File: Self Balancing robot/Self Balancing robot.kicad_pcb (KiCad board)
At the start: 2 copper layers, 90 x 60 mm, 14 parts, among them J1 TB002-500-02BE, J5 TB002-500-03BE, J7 SSK01-MPH-254-A4, J8 SSK01-MPH-254-A4, U1 ESP32-DEVKIT-V1, U2 GY-521

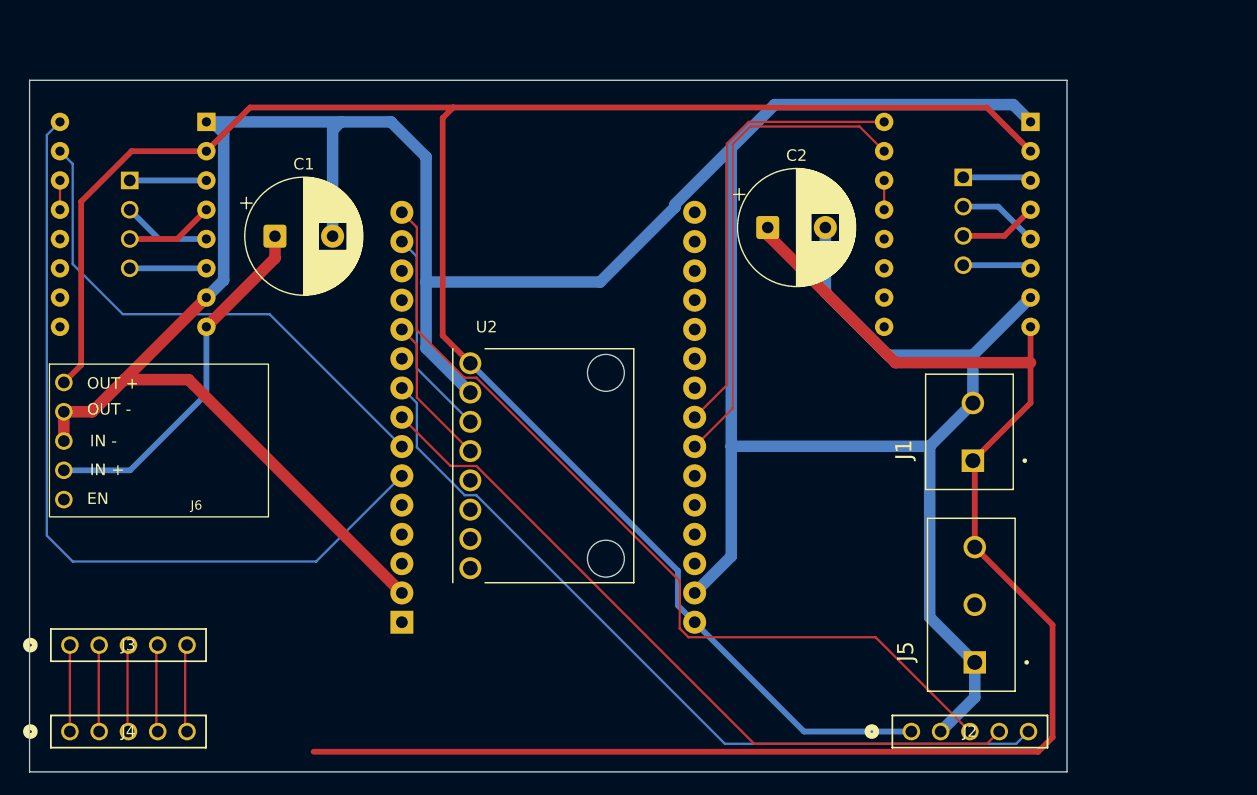
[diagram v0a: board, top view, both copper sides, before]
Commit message: In progress commit (Will fix on laptop)
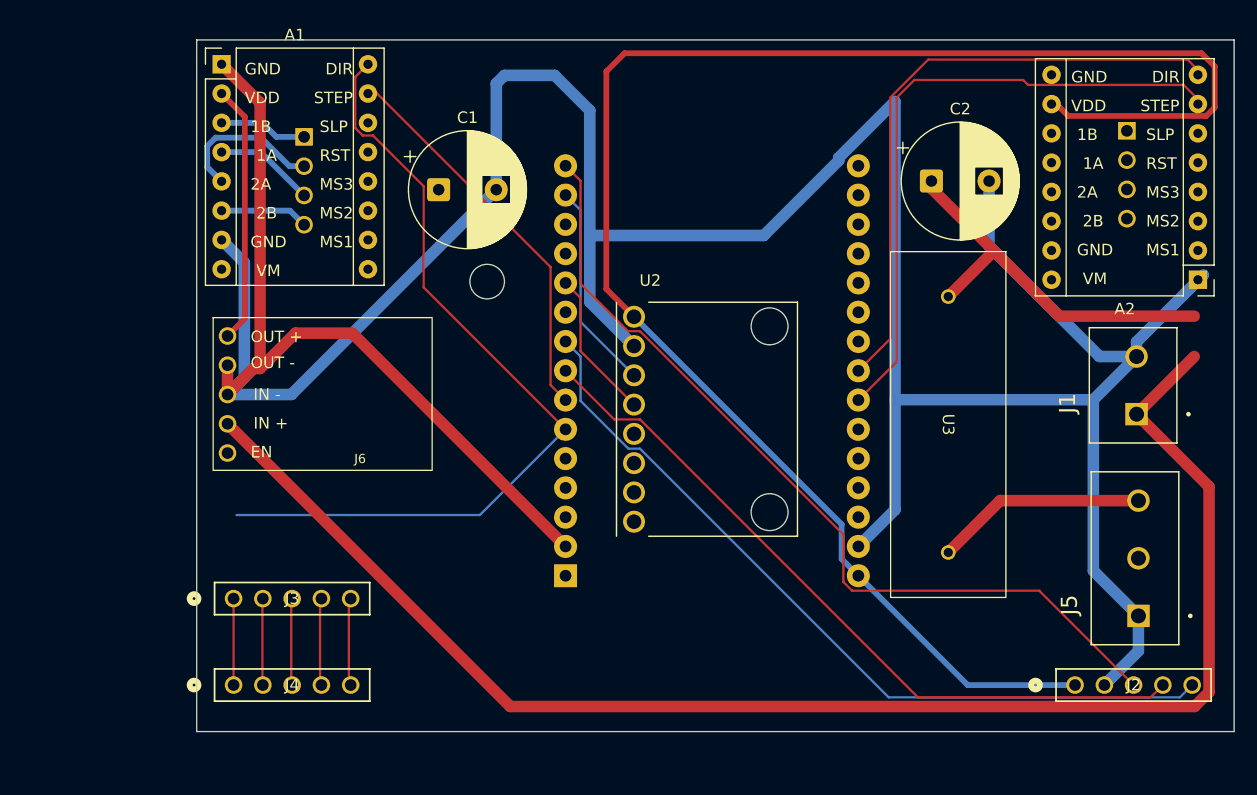
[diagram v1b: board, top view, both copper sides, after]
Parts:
- added U3: ~, 5A Fuse:5A Fuse, F.Cu at (170.2, 118.4)
- A1, A2: moved to F.Cu
- moved J7 15.6 mm to (109.3, 112.2)
- moved U2 14.8 mm to (144.3, 132.9)
- moved J3 14.8 mm to (103.2, 148.5)
- moved J4 14.8 mm to (103.2, 156.0)
- moved J6 14.8 mm to (98.2, 132.3)
- moved C1 14.8 mm to (121.0, 113.0)
- moved C2 14.8 mm to (163.7, 112.2)
- moved J8 14.8 mm to (180.7, 111.7)
- moved J1 14.8 mm to (181.5, 132.5)
- moved J2 14.8 mm to (176.2, 156.0)
- moved J5 14.8 mm to (181.7, 150.0)
- moved U1 14.8 mm to (144.7, 131.0)
- moved A1 5.17 mm to (102.2, 102.1), turned to 0 degrees
- moved A2 4.76 mm to (174.4, 102.8), turned to 0 degrees
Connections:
- J5 pad 3: +7.5V -> Net-(U3-Input)
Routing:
- net Net-(U3-Input): track 0.00 -> 18.4 mm
- net Net-(A2-DIR): track 39.3 -> 53.6 mm
- net Net-(A2-STEP): track 42.2 -> 55.4 mm
- net Net-(A1-STEP): track 45.4 -> 34.2 mm
- net +5V: track 180.4 -> 170.3 mm
- net GND: track 301.6 -> 309.3 mm
- net Net-(A2-2A): track 7.00 -> 0.00 mm
- net Net-(A2-1A): track 6.78 -> 0.00 mm
- net Net-(A2-2B): track 5.95 -> 0.00 mm
- net Net-(A2-1B): track 5.95 -> 0.00 mm
- net Net-(A1-2A): track 7.70 -> 13.3 mm
- net Net-(A2-~{RESET}): track 2.54 -> 0.00 mm
- net Net-(A1-~{RESET}): track 2.54 -> 0.00 mm
- net Net-(A1-1A): track 7.70 -> 8.71 mm
- net Net-(A1-2B): track 6.65 -> 7.66 mm
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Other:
- outline, holes or cut-outs redrawn
